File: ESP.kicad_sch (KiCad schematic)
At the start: 16 parts, among them U3 ESP32-C3-MINI-1-N4, U5 TCAN1042VDRBRQ1

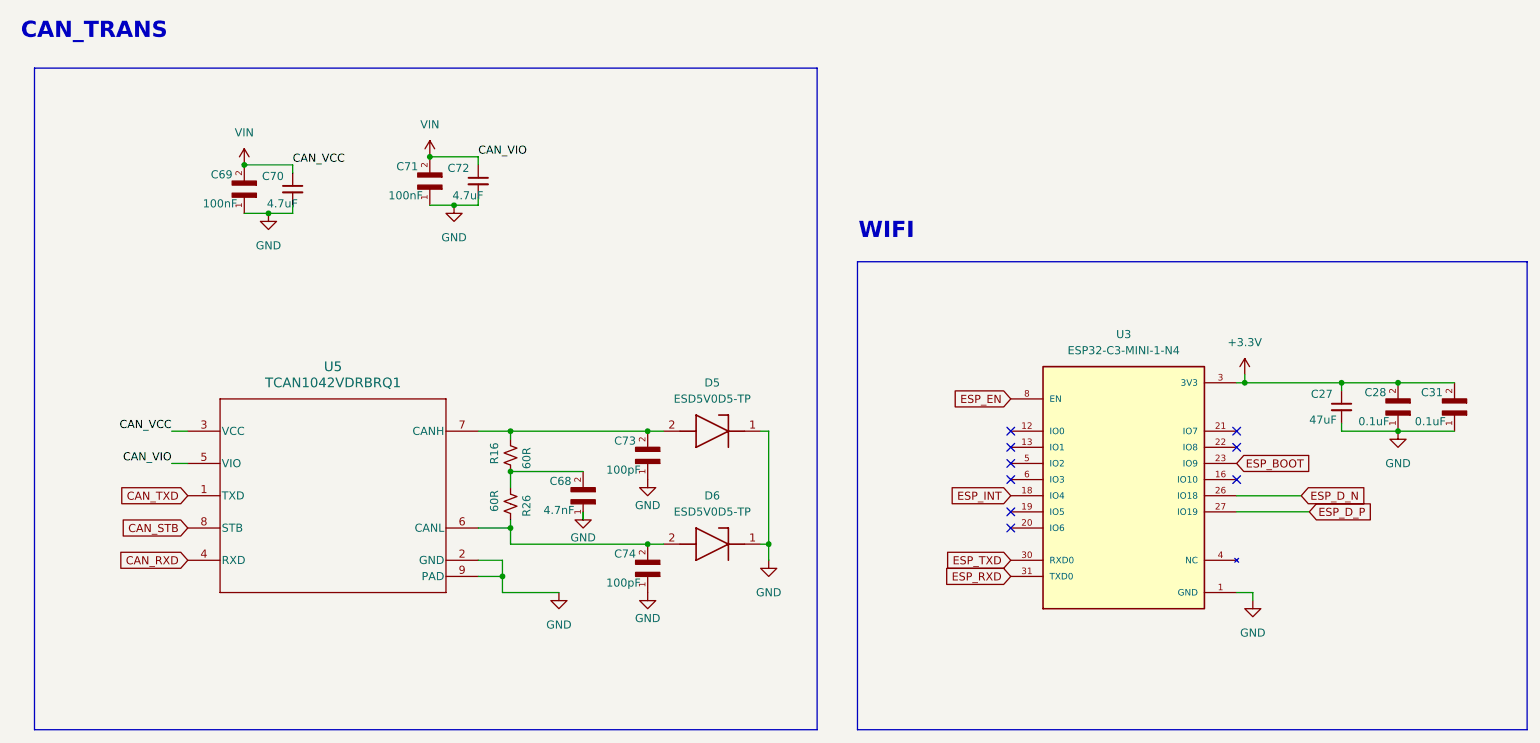
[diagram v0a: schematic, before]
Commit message: schamtic Update
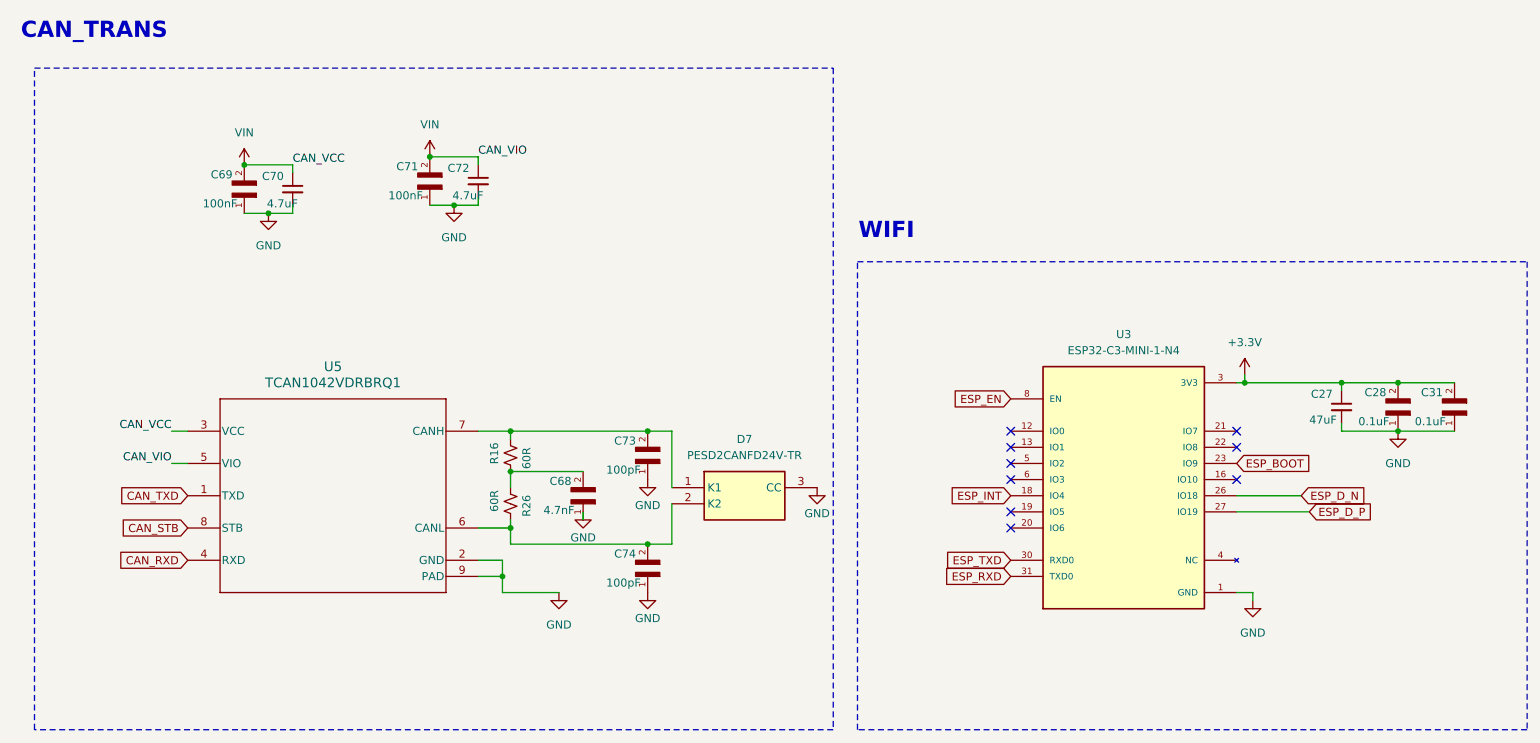
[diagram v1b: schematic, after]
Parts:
- removed D5, D6: ESD5V0D5-TP, ESD5V0D5TP, symbol ESD5V0D5-TP:ESD5V0D5-TP
- added D7: PESD2CANFD24V-TR, SOT95P230X110-3N, symbol PESD2CANFD24V-TR:PESD2CANFD24V-TR
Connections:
- net GND: now also D7.3 (CC)
- net at C74.2, R26.2, U5.6 (CANL): now also D7.2 (K2)
- net at C73.2, R16.2, U5.7 (CANH): now also D7.1 (K1)
